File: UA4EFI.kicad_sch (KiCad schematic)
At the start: 47 parts, among them J6 Conn_01x06, J7 dj7811-1, J9 USB_C, M2 Module-knock-0.2, M3 Module-vr-discrete-0.5, M4 Module-vr-max9924-0.1, M5 Module-wbo-0.5, M7 Module-can-0.1, M8 Module:mega-mcu100-f7/0.2, P3 Pad, P4 Pad, P5 Pad, P6 Pad, P7 Pad, P8 Pad, U5 JDY-33

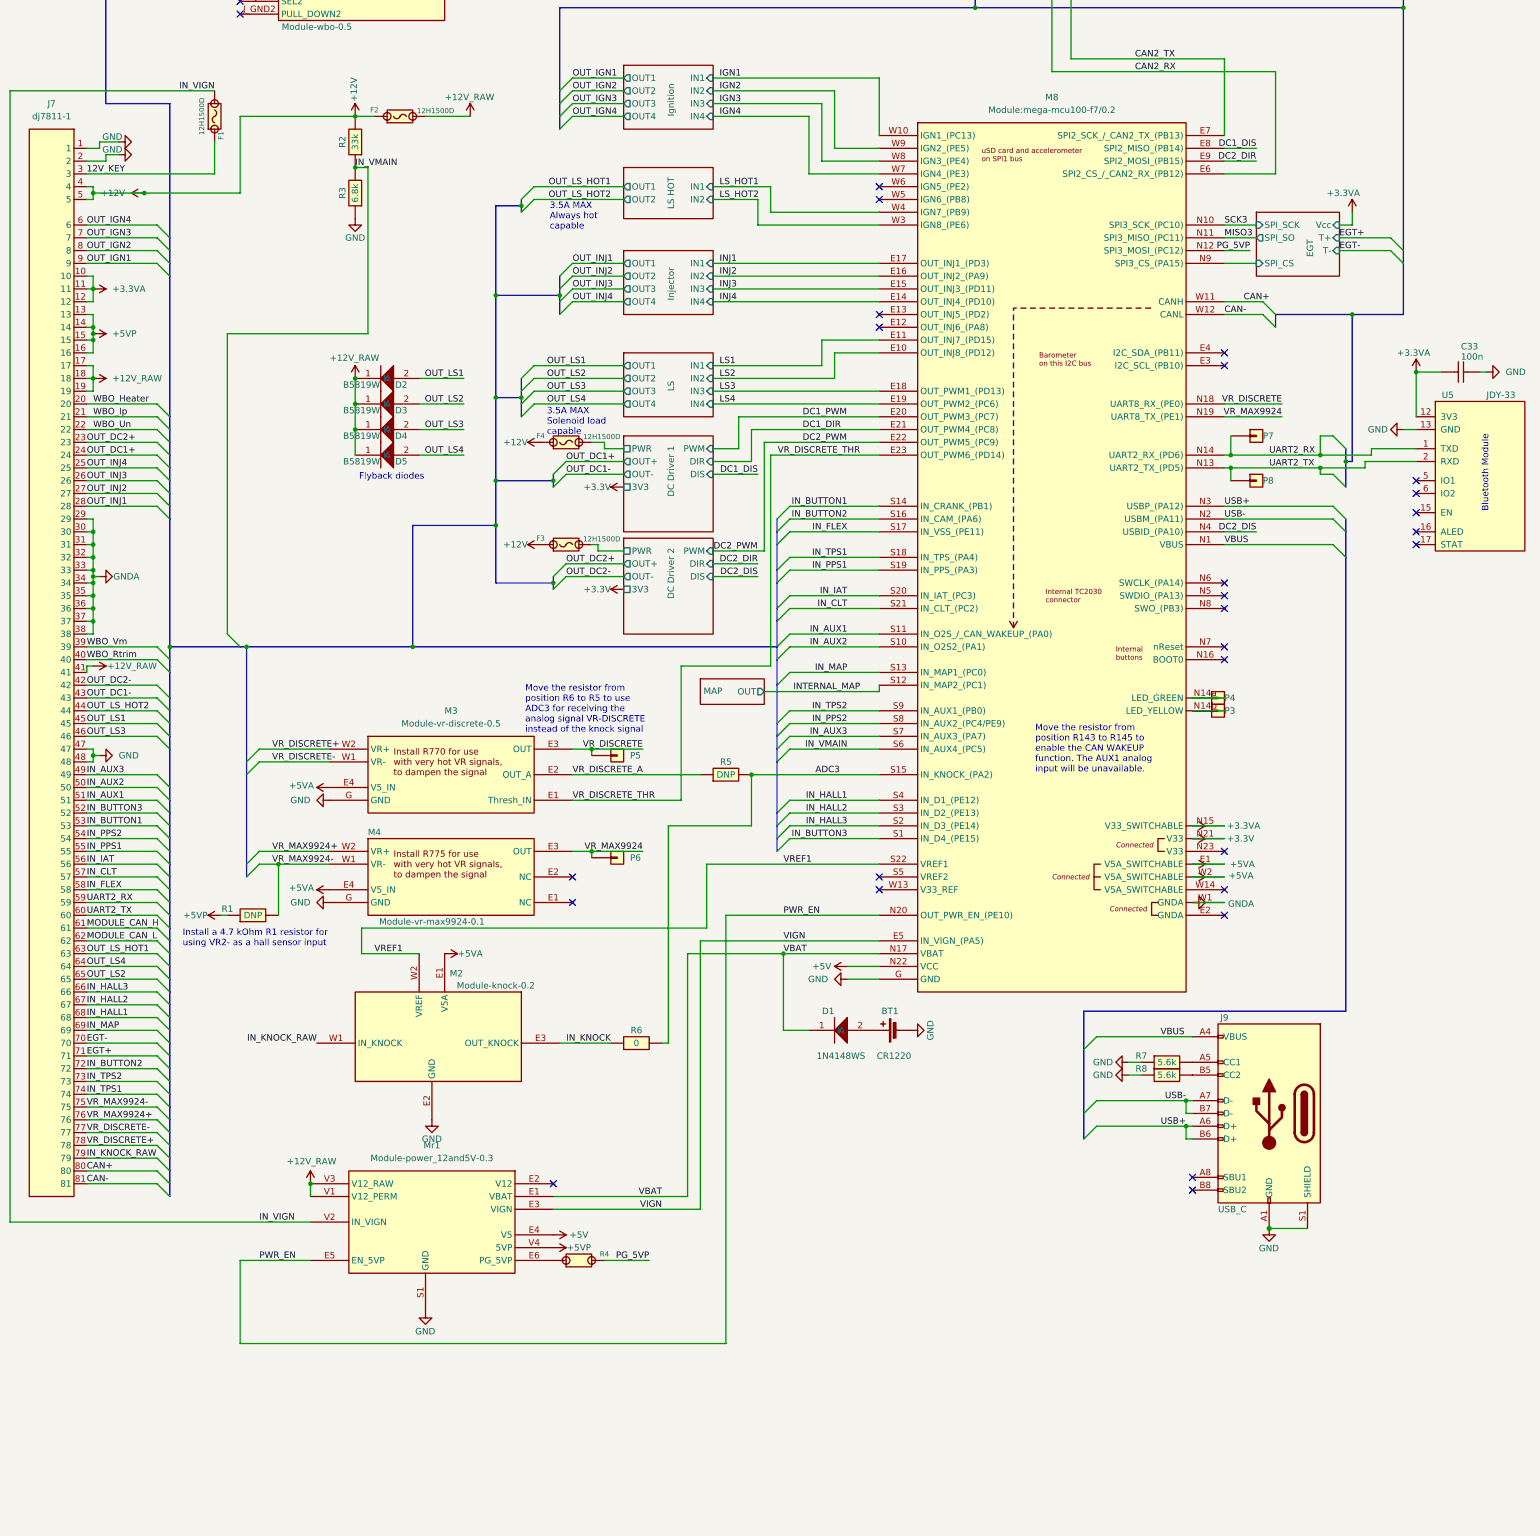
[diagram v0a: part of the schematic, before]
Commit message: update
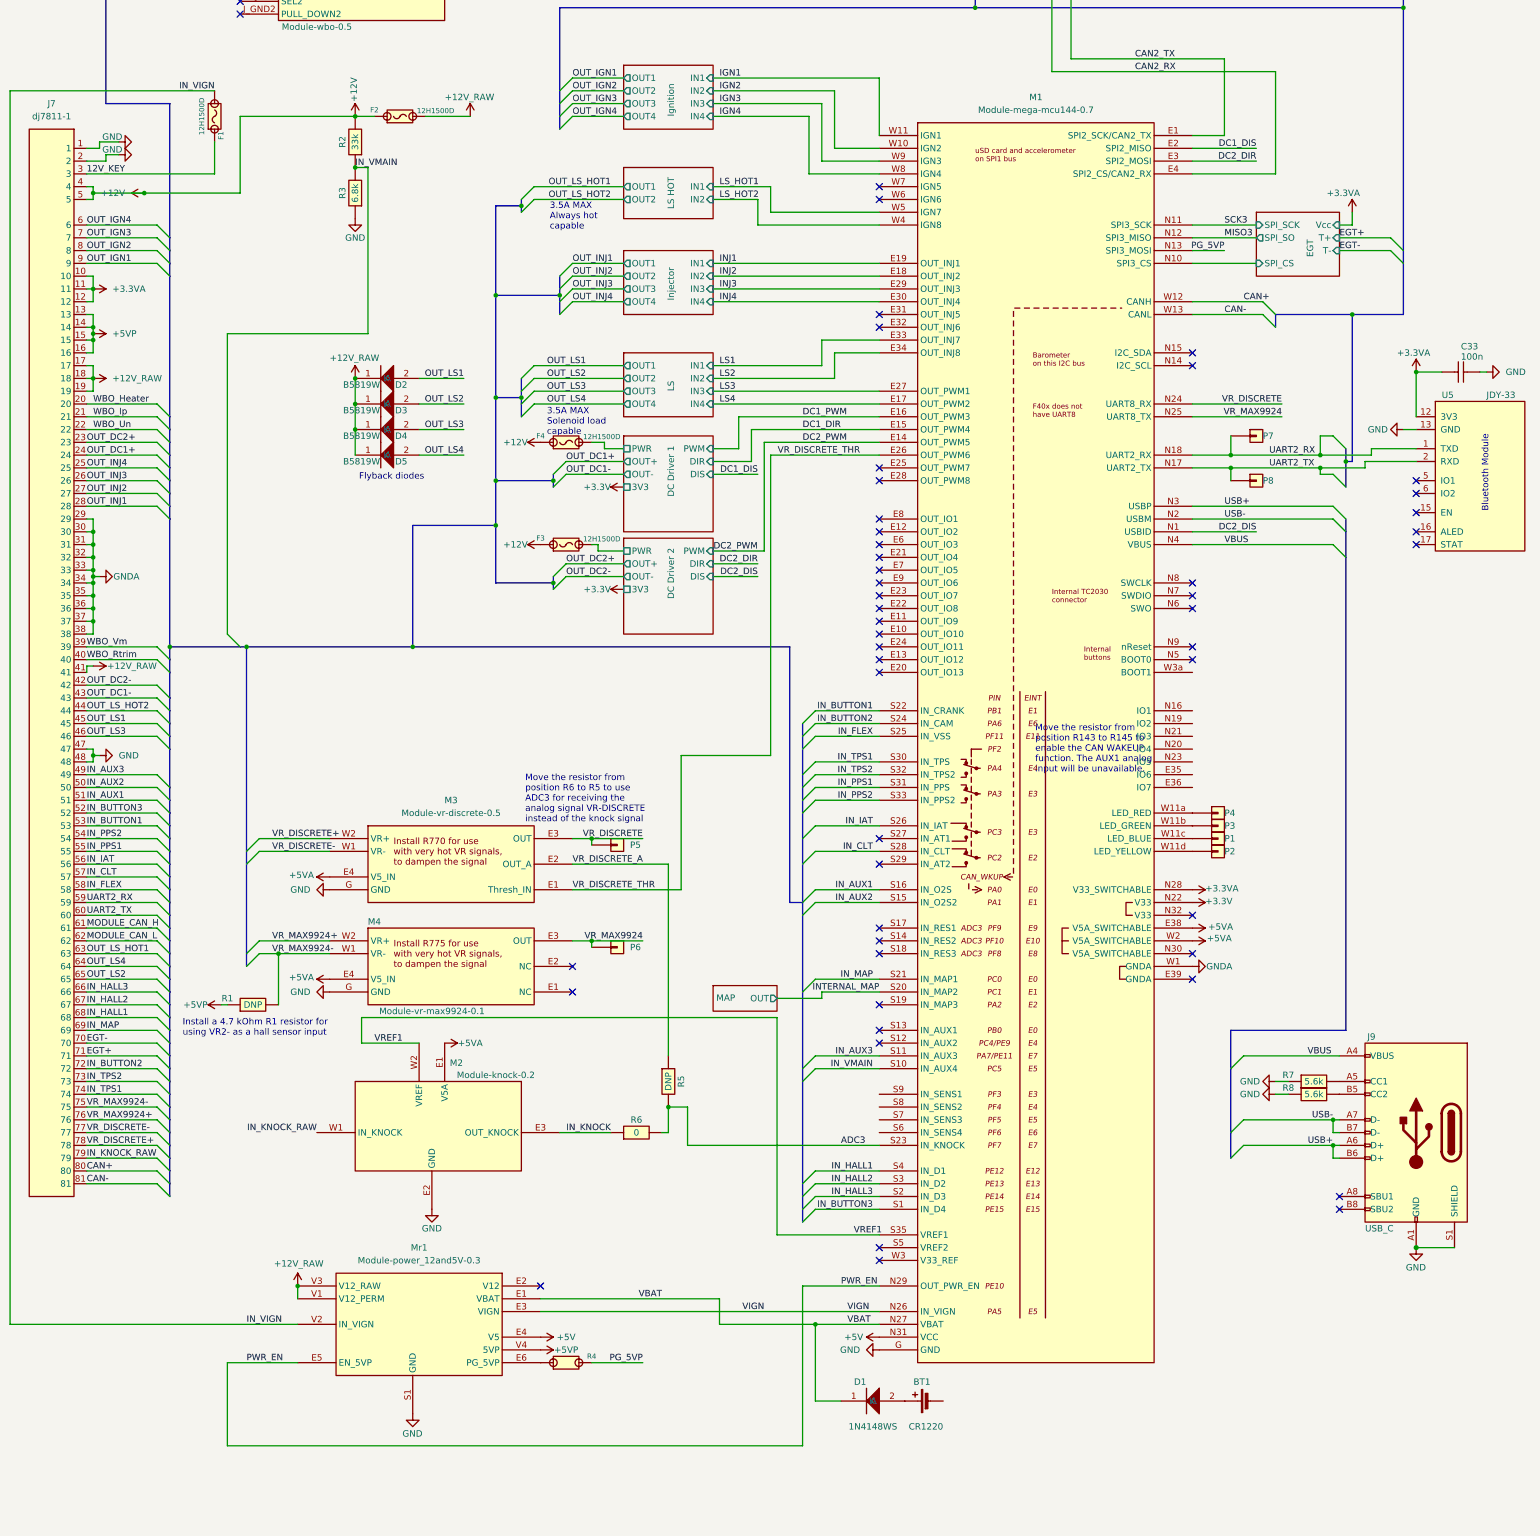
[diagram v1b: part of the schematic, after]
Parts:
- removed M8: Module:mega-mcu100-f7/0.2, mega-mcu100-f7:mega-mcu100-f7, symbol mega-mcu100-f7:Module{colon}mega-mcu100-f7/0.2
- added M1: Module-mega-mcu144-0.7, mega-mcu144:mega-mcu144, symbol mega-mcu144:Module-mega-mcu144-0.7
- added P1, P2: Pad, kicad6-libraries:PAD-TH, symbol hellen-one-common:Pad
- C33: footprint hellen-one-common:C0603 -> kicad6-libraries:C0603
- D1: footprint hellen-one-common:SOD-323 -> kicad6-libraries:SOD-323
- D2, D3, D4, D5: footprint hellen-one-common:SOD-123 -> kicad6-libraries:SOD-123
- F1, F2, F3, F4: footprint hellen-one-common:PAD-1206-PAD -> kicad6-libraries:PAD-1206-PAD
- M2: footprint hellen-one-knock-0.2:knock -> knock:knock
- M3: footprint hellen-one-vr-discrete-0.5:vr-discrete -> vr-discrete:vr-discrete
- M4: footprint hellen-one-vr-max9924-0.1:vr-max9924 -> vr-max9924:vr-max9924
- M5: footprint hellen-one-wbo-0.5:wbo -> wbo:wbo
- M7: footprint hellen-one-can-0.1:can -> can:can
- Mr1: footprint hellen-one-power_12and5V-0.3:power_12and5V -> power_12and5V:power_12and5V
- P3, P4, P5, P6, P7, P8: footprint hellen-one-common:PAD-TH -> kicad6-libraries:PAD-TH
- R1, R2, R3, R5, R6, R7, R8: footprint hellen-one-common:R0603 -> kicad6-libraries:R0603
- R35, R36, R37, R38, R39, R40: footprint hellen-one-common:R0805 -> kicad6-libraries:R0805
- R4: footprint hellen-one-common:PAD-0805-PAD -> kicad6-libraries:PAD-0805-PAD
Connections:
- net +3.3V: now also M1.N22 (V33)
- net +3.3VA: now also M1.N28 (V33_SWITCHABLE)
- net +5V: now also M1.N31 (VCC)
- net +5VA: now also M1.E38 (V5A_SWITCHABLE), M1.W2 (V5A_SWITCHABLE)
- net ADC3: now also M1.S23 (IN_KNOCK)
- net CAN+: now also M1.W12 (CANH)
- net CAN-: now also M1.W13 (CANL)
- net CAN2_RX: now also M1.E4 (SPI2_CS/CAN2_RX)
- net CAN2_TX: now also M1.E1 (SPI2_SCK/CAN2_TX)
- net DC1_DIR: now also M1.E15 (OUT_PWM4)
- net DC1_DIS: now also M1.E2 (SPI2_MISO)
- net DC1_PWM: now also M1.E16 (OUT_PWM3)
- net DC2_DIR: now also M1.E3 (SPI2_MOSI)
- net DC2_DIS: now also M1.N1 (USBID)
- net DC2_PWM: now also M1.E14 (OUT_PWM5)
- net EGT/SPI_CS: now also M1.N10 (SPI3_CS)
- net GND: now also M1.G (GND); no longer BT1.2 (-)
- net GNDA: now also M1.W1 (GNDA)
- net IGN1: now also M1.W11 (IGN1)
- net IGN2: now also M1.W10 (IGN2)
- net IGN3: now also M1.W9 (IGN3)
- net IGN4: now also M1.W8 (IGN4)
- net INJ1: now also M1.E19 (OUT_INJ1)
- net INJ2: now also M1.E18 (OUT_INJ2)
- net INJ3: now also M1.E29 (OUT_INJ3)
- net INJ4: now also M1.E30 (OUT_INJ4)
- net INTERNAL_MAP: now also M1.S20 (IN_MAP2)
- net IN_AUX1: now also M1.S16 (IN_O2S)
- net IN_AUX2: now also M1.S15 (IN_O2S2)
- net IN_AUX3: now also M1.S11 (IN_AUX3)
- net IN_BUTTON1: now also M1.S22 (IN_CRANK)
- net IN_BUTTON2: now also M1.S24 (IN_CAM)
- net IN_BUTTON3: now also M1.S1 (IN_D4)
- net IN_CLT: now also M1.S28 (IN_CLT)
- net IN_FLEX: now also M1.S25 (IN_VSS)
- net IN_HALL1: now also M1.S4 (IN_D1)
- net IN_HALL2: now also M1.S3 (IN_D2)
- net IN_HALL3: now also M1.S2 (IN_D3)
- net IN_IAT: now also M1.S26 (IN_IAT)
- net IN_MAP: now also M1.S21 (IN_MAP1)
- net IN_PPS1: now also M1.S31 (IN_PPS)
- net IN_PPS2: now also M1.S33 (IN_PPS2)
- net IN_TPS1: now also M1.S30 (IN_TPS)
- net IN_TPS2: now also M1.S32 (IN_TPS2)
- net IN_VMAIN: now also M1.S10 (IN_AUX4)
- net LS1: now also M1.E33 (OUT_INJ7)
- net LS2: now also M1.E34 (OUT_INJ8)
- net LS3: now also M1.E27 (OUT_PWM1)
- net LS4: now also M1.E17 (OUT_PWM2)
- net LS_HOT1: now also M1.W5 (IGN7)
- net LS_HOT2: now also M1.W4 (IGN8)
- net MISO3: now also M1.N12 (SPI3_MISO)
- net PG_5VP: now also M1.N13 (SPI3_MOSI)
- net PWR_EN: now also M1.N29 (OUT_PWR_EN)
- net SCK3: now also M1.N11 (SPI3_SCK)
- net UART2_RX: now also M1.N18 (UART2_RX)
- net UART2_TX: now also M1.N17 (UART2_TX)
- net USB+: now also M1.N3 (USBP)
- net USB-: now also M1.N2 (USBM)
- net VBAT: now also M1.N27 (VBAT)
- net VBUS: now also M1.N4 (VBUS)
- net VIGN: now also M1.N26 (IN_VIGN)
- net VREF1: now also M1.S35 (VREF1)
- net VR_DISCRETE: now also M1.N24 (UART8_RX)
- net VR_DISCRETE_THR: now also M1.E26 (OUT_PWM6)
- net VR_MAX9924: now also M1.N25 (UART8_TX)
- net at P4.1 (Pin_1): now also M1.W11a (LED_RED)
- net at P3.1 (Pin_1): now also M1.W11b (LED_GREEN)
- new net: M1.W11c (LED_BLUE), P1.1 (Pin_1)
- new net: M1.W11d (LED_YELLOW), P2.1 (Pin_1)
- no-connect marks 33 -> 56
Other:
- moved on the sheet: BT1, D1, J9, M2, M3, M4, Mr1, P3, P4, P5, P6, R1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
